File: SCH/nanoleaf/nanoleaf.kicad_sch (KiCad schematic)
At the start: 36 parts, among them J1 Conn_01x03_Pin, J2 Conn_01x03_Pin, J3 Conn_01x03_Pin, J7 Conn_01x05_Pin, J8 USB_C_Receptacle_USB2.0, SW1 SW_Push, SW2 SW_Push, SW3 SW_DPDT_x2, SW4 SW_DPDT_x2, SW6 SW_DPDT_x2, U1 ESP32-C3-MINI-1, U2 SN74AUP1T34DCK, U3 VEML7700-TT, U4 AMS1117CD-3.3

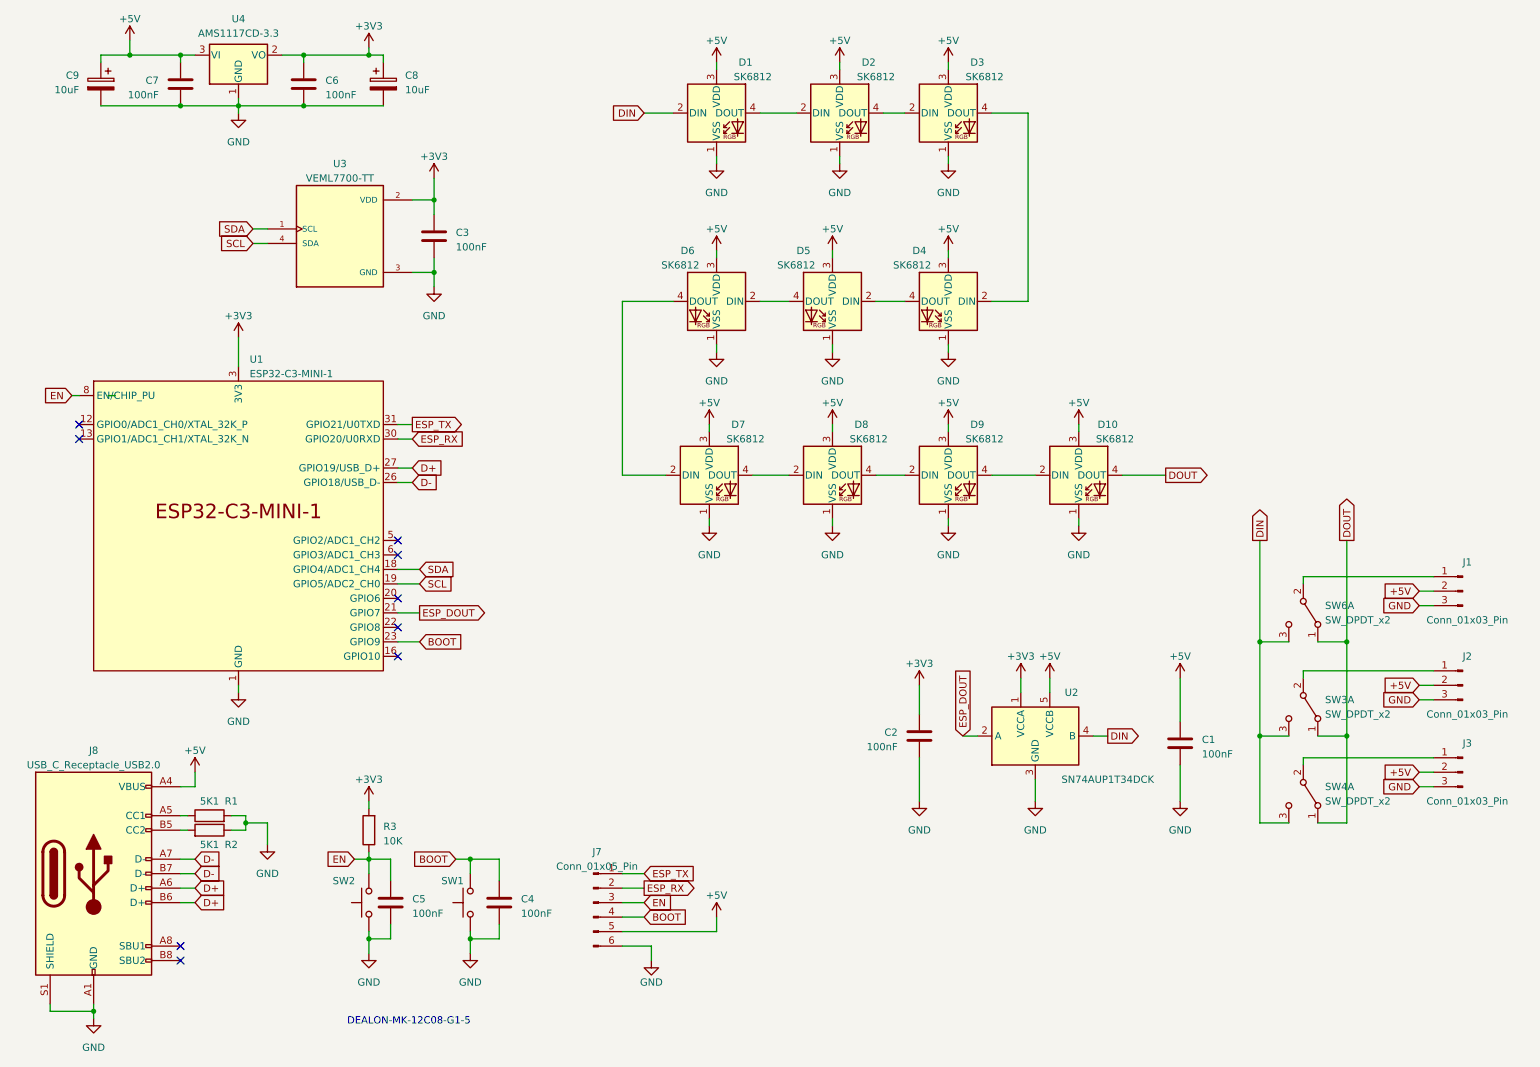
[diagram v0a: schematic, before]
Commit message: esp-c3-supermini
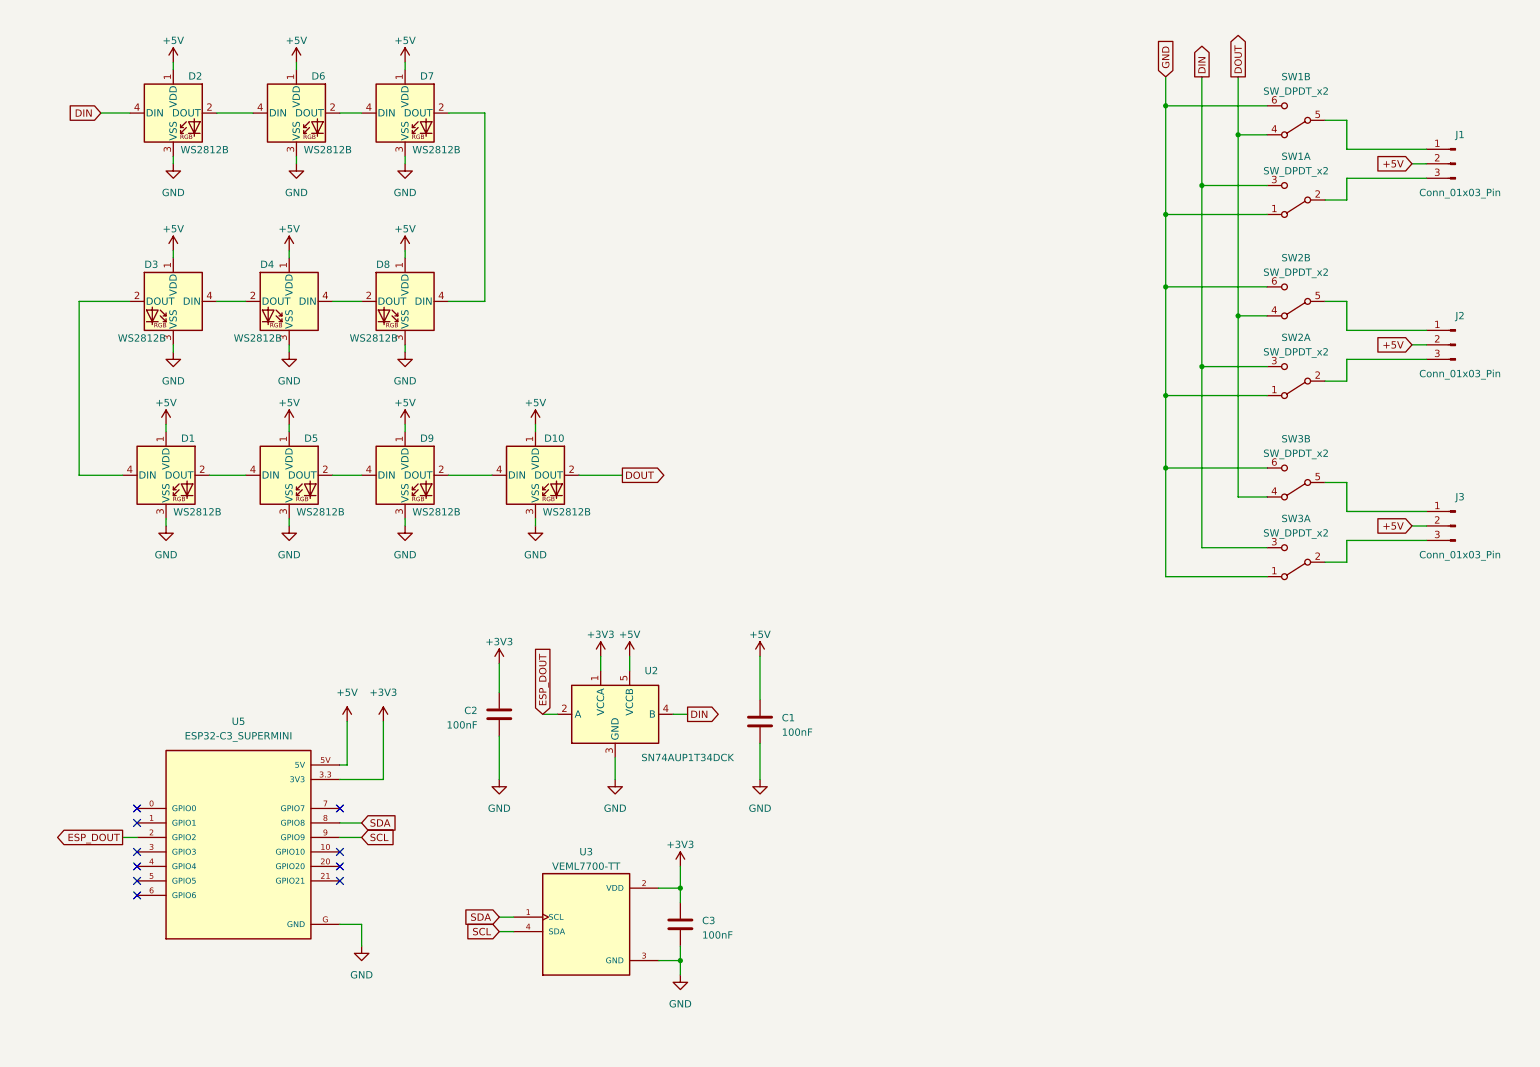
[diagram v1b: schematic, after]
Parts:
- removed C4, C5, C6, C7: 100nF, Capacitor_SMD:C_0201_0603Metric, symbol Device:C
- removed C8, C9: 10uF, Capacitor_SMD:C_Elec_3x5.4, symbol Device:C_Polarized
- removed J7: Conn_01x05_Pin, Connector_PinHeader_2.54mm:PinHeader_1x06_P2.54mm_Vertical, symbol Connector:Conn_01x06_Pin
- removed J8: USB_C_Receptacle_USB2.0, Connector_USB:USB_C_Receptacle_HRO_TYPE-C-31-M-12, symbol Connector:USB_C_Receptacle_USB2.0
- removed R1, R2: 5K1, Resistor_SMD:R_0603_1608Metric, symbol Device:R
- removed R3: 10K, Resistor_SMD:R_0603_1608Metric, symbol Device:R
- removed SW1, SW2: SW_Push, Button_Switch_SMD:SW_SPST_B3U-1000P, symbol Switch:SW_Push
- removed SW4: SW_DPDT_x2, Button_Switch_SMD:SW_DPDT_CK_JS202011JCQN, symbol Switch:SW_DPDT_x2
- removed U1: ESP32-C3-MINI-1, Espressif:ESP32-C3-MINI-1, symbol Espressif:ESP32-C3-MINI-1
- removed U4: AMS1117CD-3.3, Package_TO_SOT_SMD:TO-252-3_TabPin2, symbol Regulator_Linear:AMS1117CD-3.3
- added unit 1 of SW1
- added SW2: SW_DPDT_x2, Button_Switch_SMD:SW_DPDT_CK_JS202011JCQN, symbol Switch:SW_DPDT_x2
- added unit 2 of SW3
- added U5: ESP32-C3_SUPERMINI, Espressif:MODULE_ESP32-C3_SUPERMINI_1, symbol ESP32-C3_SUPERMINI:ESP32-C3_SUPERMINI
- D1: renamed from D7; value SK6812 -> WS2812B; footprint LED_SMD:LED_SK6812_PLCC4_5.0x5.0mm_P3.2mm -> LED_SMD:LED_WS2812B_PLCC4_5.0x5.0mm_P3.2mm; symbol LED:SK6812 -> LED:WS2812B
- D10, D9: value SK6812 -> WS2812B; footprint LED_SMD:LED_SK6812_PLCC4_5.0x5.0mm_P3.2mm -> LED_SMD:LED_WS2812B_PLCC4_5.0x5.0mm_P3.2mm; symbol LED:SK6812 -> LED:WS2812B
- D2: renamed from D1; value SK6812 -> WS2812B; footprint LED_SMD:LED_SK6812_PLCC4_5.0x5.0mm_P3.2mm -> LED_SMD:LED_WS2812B_PLCC4_5.0x5.0mm_P3.2mm; symbol LED:SK6812 -> LED:WS2812B
- D3: renamed from D6; value SK6812 -> WS2812B; footprint LED_SMD:LED_SK6812_PLCC4_5.0x5.0mm_P3.2mm -> LED_SMD:LED_WS2812B_PLCC4_5.0x5.0mm_P3.2mm; symbol LED:SK6812 -> LED:WS2812B
- D4: renamed from D5; value SK6812 -> WS2812B; footprint LED_SMD:LED_SK6812_PLCC4_5.0x5.0mm_P3.2mm -> LED_SMD:LED_WS2812B_PLCC4_5.0x5.0mm_P3.2mm; symbol LED:SK6812 -> LED:WS2812B
- D5: renamed from D8; value SK6812 -> WS2812B; footprint LED_SMD:LED_SK6812_PLCC4_5.0x5.0mm_P3.2mm -> LED_SMD:LED_WS2812B_PLCC4_5.0x5.0mm_P3.2mm; symbol LED:SK6812 -> LED:WS2812B
- D6: renamed from D2; value SK6812 -> WS2812B; footprint LED_SMD:LED_SK6812_PLCC4_5.0x5.0mm_P3.2mm -> LED_SMD:LED_WS2812B_PLCC4_5.0x5.0mm_P3.2mm; symbol LED:SK6812 -> LED:WS2812B
- D7: renamed from D3; value SK6812 -> WS2812B; footprint LED_SMD:LED_SK6812_PLCC4_5.0x5.0mm_P3.2mm -> LED_SMD:LED_WS2812B_PLCC4_5.0x5.0mm_P3.2mm; symbol LED:SK6812 -> LED:WS2812B
- D8: renamed from D4; value SK6812 -> WS2812B; footprint LED_SMD:LED_SK6812_PLCC4_5.0x5.0mm_P3.2mm -> LED_SMD:LED_WS2812B_PLCC4_5.0x5.0mm_P3.2mm; symbol LED:SK6812 -> LED:WS2812B
- J1, J2, J3: footprint Connector_JST:JST_GH_SM03B-GHS-TB_1x03-1MP_P1.25mm_Horizontal -> Connector_JST:JST_PH_B3B-PH-SM4-TB_1x03-1MP_P2.00mm_Vertical
- renumbered SW6 to SW1
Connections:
- net +3V3: now also U5.3.3 (3V3)
- net +5V: now also D1.1 (VDD), D10.1 (VDD), D2.1 (VDD), D3.1 (VDD), D4.1 (VDD), D5.1 (VDD), D6.1 (VDD), D7.1 (VDD), D8.1 (VDD), D9.1 (VDD), U5.5V; no longer D1.3 (VDD), D10.3 (VDD), D2.3 (VDD), D3.3 (VDD), D4.3 (VDD), D5.3 (VDD), D6.3 (VDD), D7.3 (VDD), D8.3 (VDD), D9.3 (VDD)
- net DIN: now also D2.4 (DIN), SW1.3 (C), SW2.3 (C); no longer D2.2 (DIN), SW1.3 (C)
- net DOUT: now also D10.2 (DOUT), SW1.4 (A), SW2.4 (A), SW3.4 (A); no longer D10.4 (DOUT), SW1.1 (A), SW3.1 (A)
- net ESP_DOUT: now also U5.2 (GPIO2)
- net GND: now also D1.3 (VSS), D10.3 (VSS), D2.3 (VSS), D3.3 (VSS), D4.3 (VSS), D5.3 (VSS), D6.3 (VSS), D7.3 (VSS), D8.3 (VSS), D9.3 (VSS), SW1.6 (C), SW3.1 (A), SW1.1 (A), SW2.1 (A), SW2.6 (C), SW3.6 (C), U5.G (GND); no longer D1.1 (VSS), D10.1 (VSS), D2.1 (VSS), D3.1 (VSS), D4.1 (VSS), D5.1 (VSS), D6.1 (VSS), D7.1 (VSS), D8.1 (VSS), D9.1 (VSS), J1.3 (Pin_3), J2.3 (Pin_3), J3.3 (Pin_3)
- net SCL: now also U5.9 (GPIO9)
- net SDA: now also U5.8 (GPIO8)
- net at D3.2 (DOUT): now also D1.4 (DIN); no longer D4.4 (DOUT)
- net at D3.4 (DIN): now also D4.2 (DOUT); no longer D1.2 (DIN)
- net at J1.1 (Pin_1): now also SW1.5 (B); no longer SW1.2 (B)
- net at D5.2 (DOUT): now also D9.4 (DIN); no longer D1.4 (DOUT)
- net at D8.4 (DIN): now also D7.2 (DOUT); no longer D4.2 (DIN)
- net at D5.4 (DIN): now also D1.2 (DOUT); no longer D9.2 (DIN)
- net at D6.2 (DOUT): now also D7.4 (DIN); no longer D2.4 (DOUT)
- net at SW3.2 (B): now also J3.3 (Pin_3); no longer J2.1 (Pin_1)
- net at D6.4 (DIN): now also D2.2 (DOUT); no longer D7.2 (DIN)
- net at D8.2 (DOUT): now also D4.4 (DIN); no longer D7.4 (DOUT)
- net at J3.1 (Pin_1): now also SW3.5 (B)
- new net: J1.3 (Pin_3), SW1.2 (B)
- new net: J2.3 (Pin_3), SW2.2 (B)
- new net: D10.4 (DIN), D9.2 (DOUT)
- new net: J2.1 (Pin_1), SW2.5 (B)
- no-connect marks 9 -> 10
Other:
- note removed: "DEALON-MK-12C08-G1-5"
- moved on the sheet: C1, C2, C3, D1, D10, D2, D3, D4, D5, D6, D7, D8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

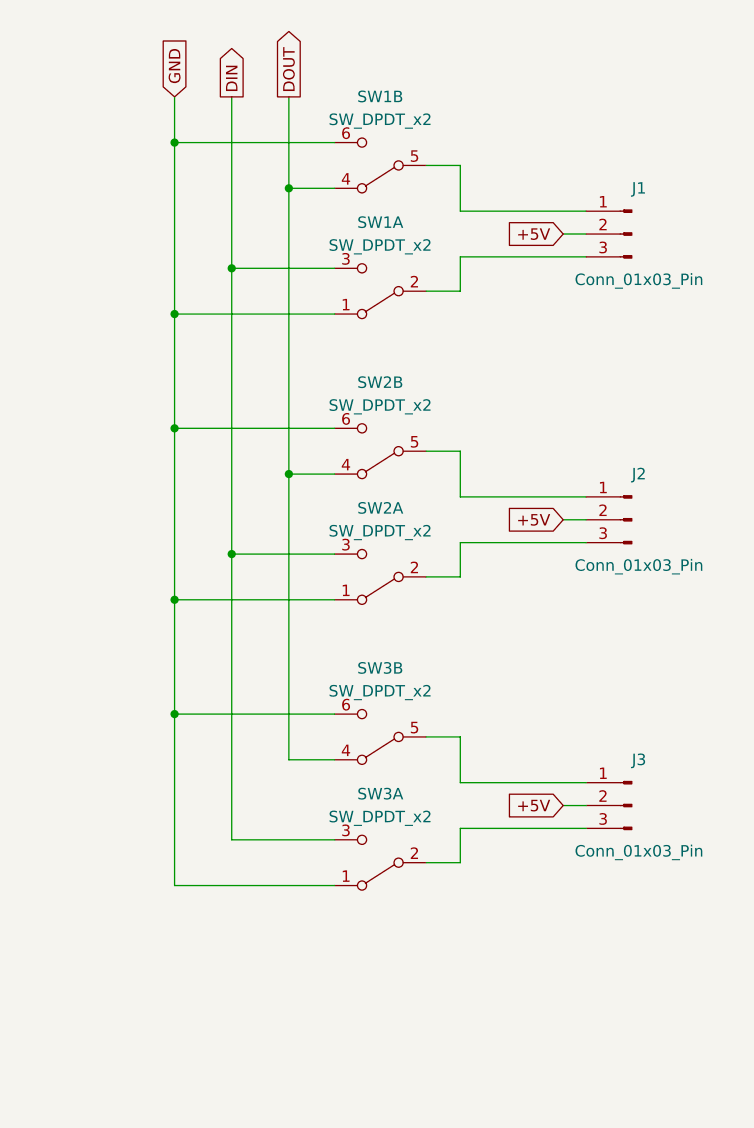
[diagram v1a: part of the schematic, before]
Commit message: switch and jst PH
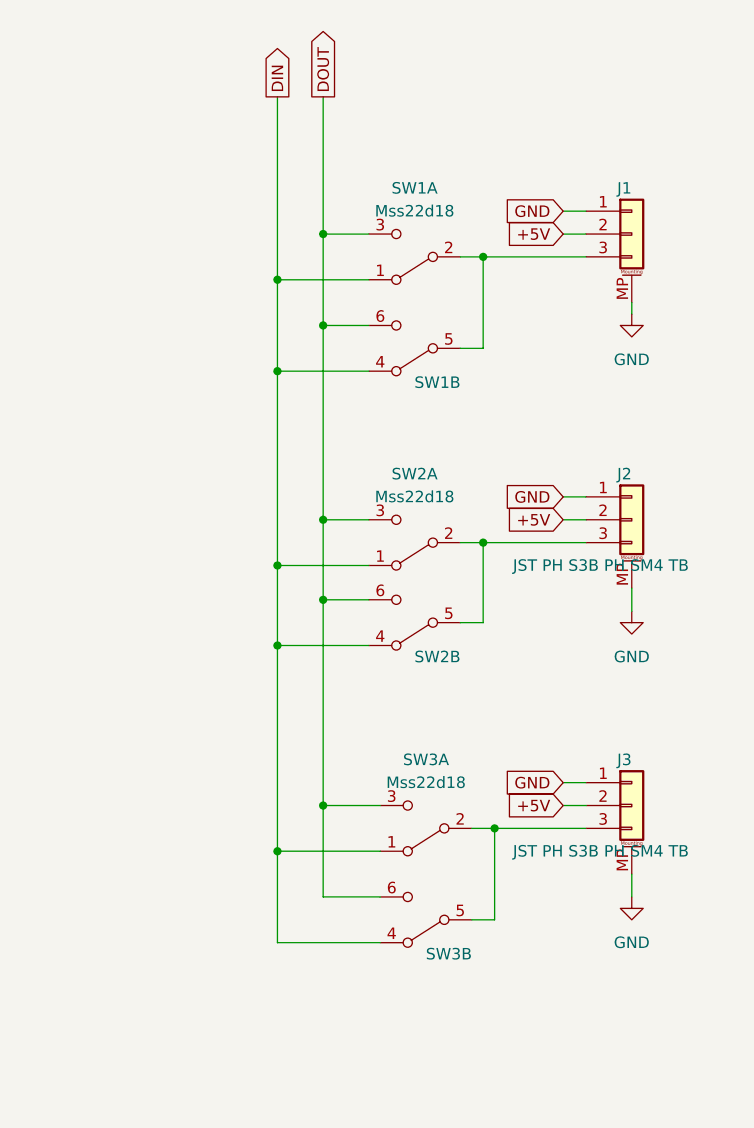
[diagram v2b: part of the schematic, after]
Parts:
- C1, C2, C3: footprint Capacitor_SMD:C_0201_0603Metric -> Capacitor_SMD:C_0603_1608Metric
- J1, J2, J3: value Conn_01x03_Pin -> JST PH S3B PH SM4 TB; footprint Connector_JST:JST_PH_B3B-PH-SM4-TB_1x03-1MP_P2.00mm_Vertical -> Connector_JST:JST_PH_S3B-PH-SM4-TB_1x03-1MP_P2.00mm_Horizontal; symbol Connector:Conn_01x03_Pin -> Connector_Generic_MountingPin:Conn_01x03_MountingPin
- SW1, SW2, SW3: value SW_DPDT_x2 -> Mss22d18; footprint Button_Switch_SMD:SW_DPDT_CK_JS202011JCQN -> Button_Switch_SMD:SW_DPDT_CK_JS202011SCQN
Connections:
- net DIN: now also SW1.1 (A), SW1.4 (A), SW2.1 (A), SW2.4 (A), SW3.1 (A), SW3.4 (A); no longer SW1.3 (C), SW2.3 (C), SW3.3 (C)
- net DOUT: now also SW1.3 (C), SW1.6 (C), SW2.3 (C), SW2.6 (C), SW3.3 (C), SW3.6 (C); no longer SW1.4 (A), SW2.4 (A), SW3.4 (A)
- net GND: now also J1.1 (Pin_1), J1.MP (MountPin), J2.1 (Pin_1), J2.MP (MountPin), J3.1 (Pin_1), J3.MP (MountPin); no longer SW1.1 (A), SW1.6 (C), SW2.1 (A), SW2.6 (C), SW3.1 (A), SW3.6 (C)
- net at SW1.5 (B): now also J1.3 (Pin_3), SW1.2 (B); no longer J1.1 (Pin_1)
- net at SW3.5 (B): now also J3.3 (Pin_3), SW3.2 (B); no longer J3.1 (Pin_1)
- net at J2.3 (Pin_3), SW2.2 (B): now also SW2.5 (B)
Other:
- moved on the sheet: J1, J2, J3, SW1A, SW2A, SW3A
